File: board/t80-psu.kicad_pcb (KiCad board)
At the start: 2 copper layers, 26 x 80 mm, 28 parts, among them J1 Conn_01x02_Female, U1 FR8205, U2 FR8205

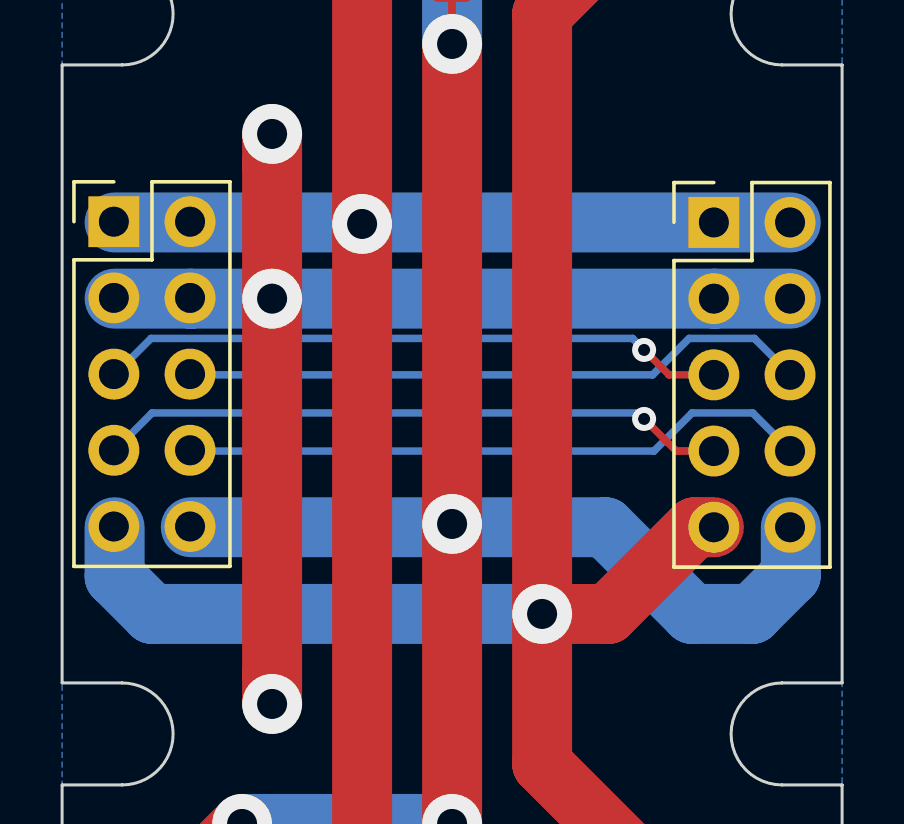
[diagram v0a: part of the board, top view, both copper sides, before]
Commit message: WIP
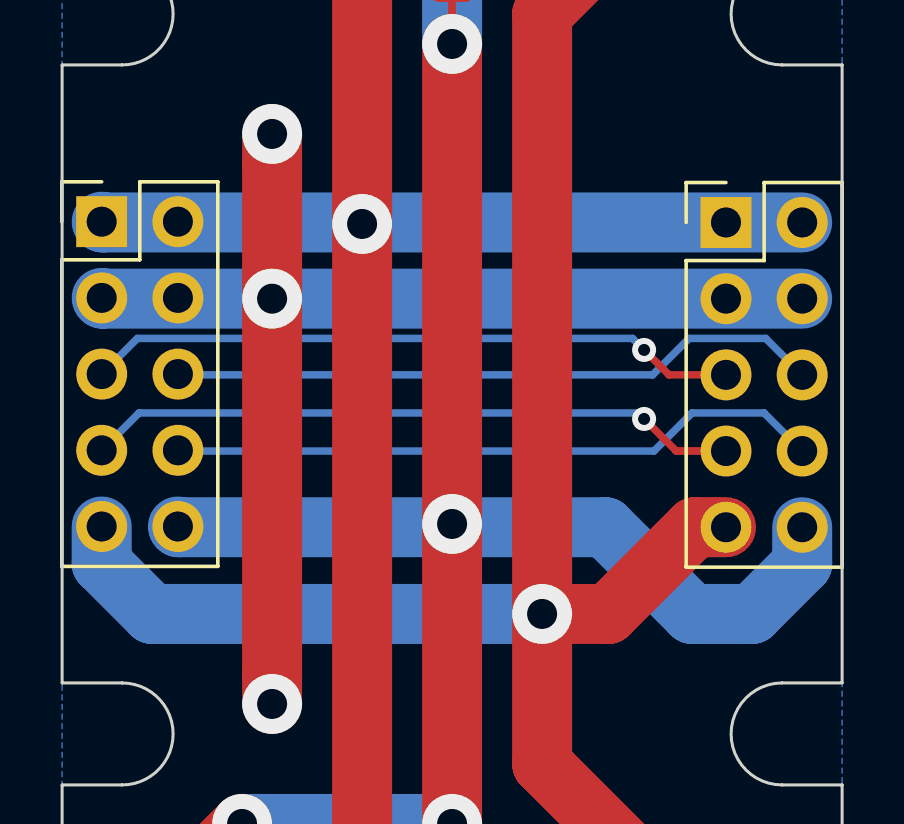
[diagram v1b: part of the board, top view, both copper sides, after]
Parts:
- moved X1 0.41 mm to (86.3, 94.9)
- moved X2 0.41 mm to (107.1, 95.0)
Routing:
- net /SDA: track 21.0 -> 21.8 mm
- net /PWR_LINE_12V: track 22.5 -> 23.4 mm
- net /IRQ: track 21.1 -> 21.9 mm
- net /PWR_LINE_GND: track 22.5 -> 23.4 mm
- net /RST: track 21.0 -> 21.9 mm
- net /SCL: track 21.0 -> 21.8 mm
- net /PWR_LINE_5V: track 23.3 -> 23.9 mm
- net /PWR_LINE_3V3: track 23.3 -> 23.9 mm
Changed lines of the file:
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@@
   )
   (footprint "Connector_PinHeader_2.54mm:PinHeader_2x05_P2.54mm_Vertical" locked (layer "F.Cu")
-    (at 106.725 94.95)
+    (at 107.13 94.95)
     (descr "Through hole straight pin header, 2x05, 2.54mm pitch, double rows")
     (tags "Through hole pin header THT 2x05 2.54mm double row")
@@
   )
   (footprint "Connector_PinHeader_2.54mm:PinHeader_2x05_P2.54mm_Vertical" locked (layer "F.Cu")
-    (at 86.725 94.925)
+    (at 86.32 94.925)
     (descr "Through hole straight pin header, 2x05, 2.54mm pitch, double rows")
     (tags "Through hole pin header THT 2x05 2.54mm double row")
@@
     (style (thickness 0.15) (arrow_length 1.27) (text_position_mode 0) (extension_height 0.58642) (extension_offset 0.5) keep_text_aligned)
   )
-  (segment (start 105.23 100.03) (end 106.75 100.03) (width 0.25) (layer "F.Cu") (net 1))
   (segment (start 104.4 99.2) (end 105.23 100.03) (width 0.25) (layer "F.Cu") (net 1))
+  (segment (start 105.23 100.03) (end 107.13 100.03) (width 0.25) (layer "F.Cu") (net 1))
   (via (at 104.4 99.2) (size 0.8) (drill 0.4) (layers "F.Cu" "B.Cu") (net 1))
+  (segment (start 86.32 100.005) (end 87.51 98.815) (width 0.25) (layer "B.Cu") (net 1))
   (segment (start 104.015 98.815) (end 104.4 99.2) (width 0.25) (layer "B.Cu") (net 1))
-  (segment (start 86.75 100.03) (end 87.965 98.815) (width 0.25) (layer "B.Cu") (net 1))
-  (segment (start 104.015 98.815) (end 87.965 98.815) (width 0.25) (layer "B.Cu") (net 1))
+  (segment (start 87.51 98.815) (end 104.015 98.815) (width 0.25) (layer "B.Cu") (net 1))
+  (segment (start 108.455 98.815) (end 109.67 100.03) (width 0.25) (layer "B.Cu") (net 2))
+  (segment (start 88.86 100.005) (end 88.885 100.03) (width 0.25) (layer "B.Cu") (net 2))
+  (segment (start 105.9 98.815) (end 108.455 98.815) (width 0.25) (layer "B.Cu") (net 2))
+  (segment (start 88.885 100.03) (end 104.685 100.03) (width 0.25) (layer "B.Cu") (net 2))
   (segment (start 104.685 100.03) (end 105.9 98.815) (width 0.25) (layer "B.Cu") (net 2))
-  (segment (start 108.075 98.815) (end 109.29 100.03) (width 0.25) (layer "B.Cu") (net 2))
-  (segment (start 105.9 98.815) (end 108.075 98.815) (width 0.25) (layer "B.Cu") (net 2))
-  (segment (start 104.685 100.03) (end 89.29 100.03) (width 0.25) (layer "B.Cu") (net 2))
   (segment (start 104.4 101.5) (end 105.47 102.57) (width 0.25) (layer "F.Cu") (net 3))
-  (segment (start 105.47 102.57) (end 106.75 102.57) (width 0.25) (layer "F.Cu") (net 3))
+  (segment (start 105.47 102.57) (end 107.13 102.57) (width 0.25) (layer "F.Cu") (net 3))
   (via (at 104.4 101.5) (size 0.8) (drill 0.4) (layers "F.Cu" "B.Cu") (net 3))
   (segment (start 104.4 101.5) (end 104.2 101.3) (width 0.25) (layer "B.Cu") (net 3))
-  (segment (start 88 101.3) (end 104.2 101.3) (width 0.25) (layer "B.Cu") (net 3))
-  (segment (start 88 101.3) (end 86.75 102.55) (width 0.25) (layer "B.Cu") (net 3))
-  (segment (start 106 101.3) (end 108.02 101.3) (width 0.25) (layer "B.Cu") (net 4))
-  (segment (start 108.02 101.3) (end 109.29 102.57) (width 0.25) (layer "B.Cu") (net 4))
+  (segment (start 104.2 101.3) (end 87.565 101.3) (width 0.25) (layer "B.Cu") (net 3))
+  (segment (start 87.565 101.3) (end 86.32 102.545) (width 0.25) (layer "B.Cu") (net 3))
+  (segment (start 88.86 102.545) (end 88.885 102.57) (width 0.25) (layer "B.Cu") (net 4))
+  (segment (start 88.885 102.57) (end 104.73 102.57) (width 0.25) (layer "B.Cu") (net 4))
   (segment (start 104.73 102.57) (end 106 101.3) (width 0.25) (layer "B.Cu") (net 4))
-  (segment (start 104.73 102.57) (end 89.29 102.57) (width 0.25) (layer "B.Cu") (net 4))
+  (segment (start 108.4 101.3) (end 109.67 102.57) (width 0.25) (layer "B.Cu") (net 4))
+  (segment (start 106 101.3) (end 108.4 101.3) (width 0.25) (layer "B.Cu") (net 4))
   (via (at 95 95) (size 2) (drill 1) (layers "F.Cu" "B.Cu") (net 5))
-  (segment (start 109.29 94.95) (end 95.05 94.95) (width 2) (layer "B.Cu") (net 5))
-  (segment (start 95.05 94.95) (end 86.75 94.95) (width 2) (layer "B.Cu") (net 5))
+  (segment (start 109.67 94.95) (end 86.345 94.95) (width 2) (layer "B.Cu") (net 5))
+  (segment (start 86.345 94.95) (end 86.32 94.925) (width 2) (layer "B.Cu") (net 5))
   (via (at 92 97.49) (size 2) (drill 1) (layers "F.Cu" "B.Cu") (net 6))
-  (segment (start 106.75 97.49) (end 89.29 97.49) (width 2) (layer "B.Cu") (net 6))
-  (segment (start 109.29 97.49) (end 106.75 97.49) (width 2) (layer "B.Cu") (net 6))
-  (segment (start 89.29 97.49) (end 86.75 97.49) (width 2) (layer "B.Cu") (net 6))
-  (segment (start 106.725 105.11) (end 106.09 105.11) (width 2) (layer "F.Cu") (net 7))
+  (segment (start 86.345 97.49) (end 86.32 97.465) (width 2) (layer "B.Cu") (net 6))
+  (segment (start 109.67 97.49) (end 86.345 97.49) (width 2) (layer "B.Cu") (net 6))
   (segment (start 103.2 108) (end 101 108) (width 2) (layer "F.Cu") (net 7))
   (segment (start 106.09 105.11) (end 103.2 108) (width 2) (layer "F.Cu") (net 7))
+  (segment (start 107.13 105.11) (end 106.09 105.11) (width 2) (layer "F.Cu") (net 7))
   (via (at 101 108) (size 2) (drill 1) (layers "F.Cu" "B.Cu") (net 7))
-  (segment (start 88 108) (end 86.75 106.75) (width 2) (layer "B.Cu") (net 7))
+  (segment (start 88 108) (end 86.32 106.32) (width 2) (layer "B.Cu") (net 7))
   (segment (start 101 108) (end 88 108) (width 2) (layer "B.Cu") (net 7))
-  (segment (start 86.75 106.75) (end 86.75 105.11) (width 2) (layer "B.Cu") (net 7))
+  (segment (start 86.32 106.32) (end 86.32 105.085) (width 2) (layer "B.Cu") (net 7))
   (via (at 98 105) (size 2) (drill 1) (layers "F.Cu" "B.Cu") (net 8))
-  (segment (start 109.29 106.71) (end 109.29 105.11) (width 2) (layer "B.Cu") (net 8))
+  (segment (start 88.885 105.11) (end 103.11 105.11) (width 2) (layer "B.Cu") (net 8))
+  (segment (start 103.11 105.11) (end 106 108) (width 2) (layer "B.Cu") (net 8))
+  (segment (start 108 108) (end 109.67 106.33) (width 2) (layer "B.Cu") (net 8))
+  (segment (start 109.67 106.33) (end 109.67 105.11) (width 2) (layer "B.Cu") (net 8))
+  (segment (start 88.86 105.085) (end 88.885 105.11) (width 2) (layer "B.Cu") (net 8))
   (segment (start 106 108) (end 108 108) (width 2) (layer "B.Cu") (net 8))
-  (segment (start 108 108) (end 109.29 106.71) (width 2) (layer "B.Cu") (net 8))
-  (segment (start 89.29 105.11) (end 103.11 105.11) (width 2) (layer "B.Cu") (net 8))
-  (segment (start 103.11 105.11) (end 106 108) (width 2) (layer "B.Cu") (net 8))
   (segment (start 100.04 135.96) (end 100.04 134.049999) (width 2) (layer "F.Cu") (net 9))
   (segment (start 98 78) (end 98 74) (width 2) (layer "F.Cu") (net 9))
